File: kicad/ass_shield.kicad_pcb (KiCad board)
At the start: 2 copper layers, 80 x 80 mm, 151 parts, among them J1 6-40V, J2 DEBUG, J3 5V, J4 UART2, J5 U.FL, J6 i2s, J7 SP, J8 U.FL, M1 CR1220SMD, Q1 BC817, U1 OPiZero, U2 DS3231M, U3 24LC256, U4 nRF24L01P, U5 PCF8574, U6 CC2530F, X1 USB_F1, X2 USB_F1, Y1 9,84375 MHz, Y2 13,5600 MHz, Y3 4,8970 MHz, Y4 6,7458 MHz, Y5 32 MHz, Y6 16 MHz, Y7 32 MHz

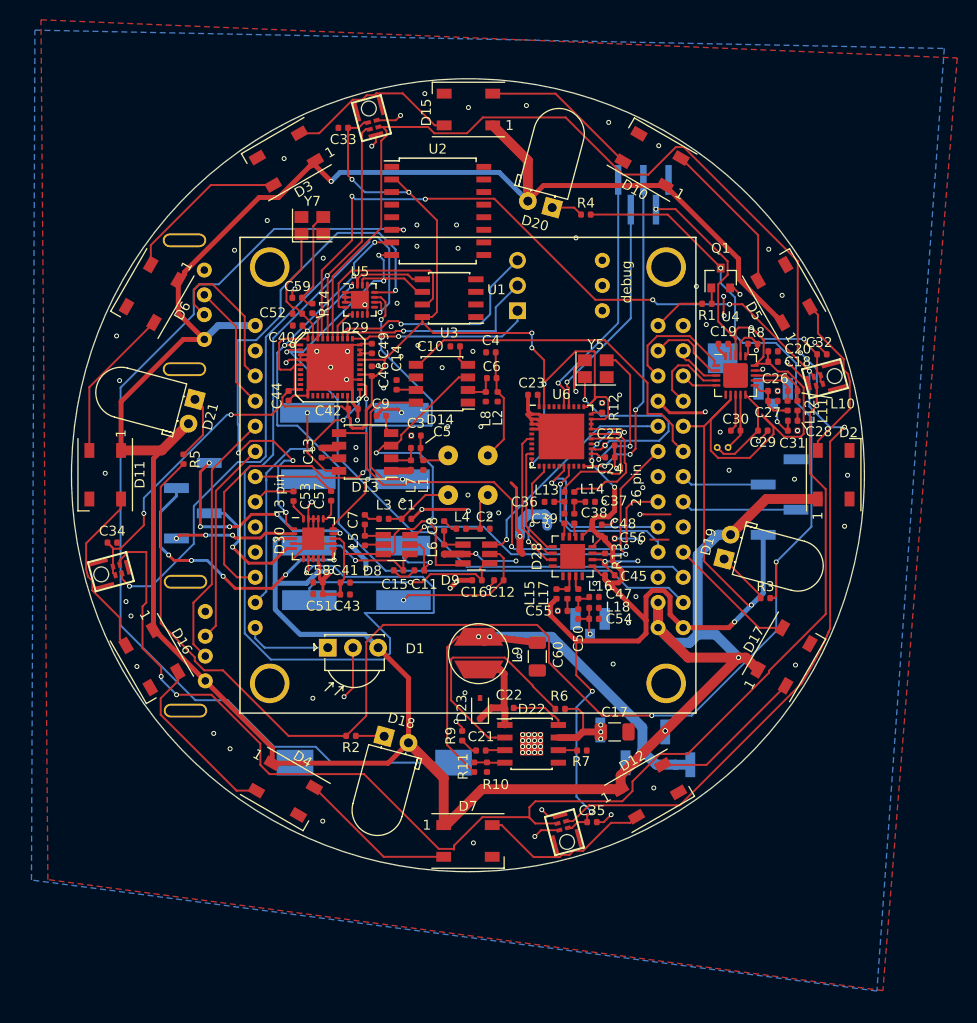
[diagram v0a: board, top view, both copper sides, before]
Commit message: a msg
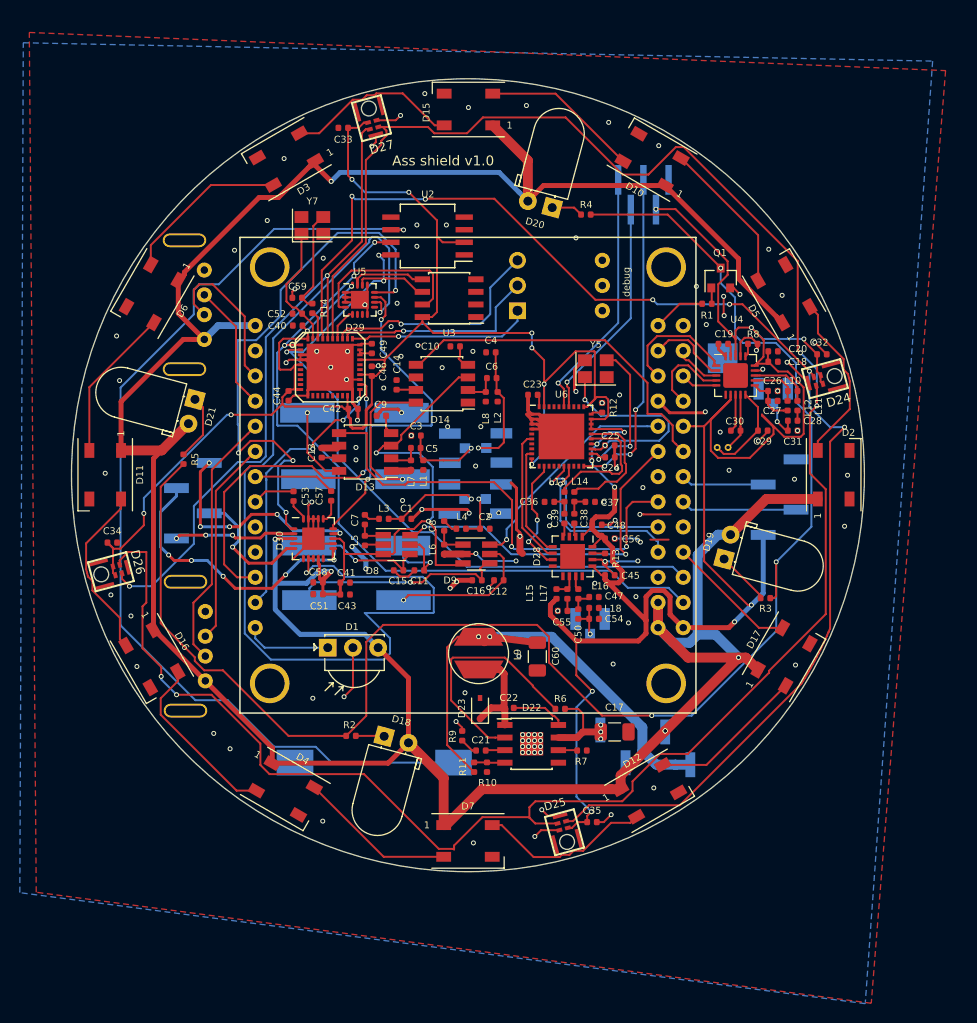
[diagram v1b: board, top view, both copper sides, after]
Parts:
- AE1, AE2, AE3, AE4: footprint imm:rf_antenna_0.8mm -> Connector_Coaxial:U.FL_Hirose_U.FL-R-SMT-1_Vertical; moved to B.Cu
- C10, C9: value 0,047 µF -> 47 nF
- C17: value 10µF 50V -> 10 µF 50V
- C22: value 100 nF -> 0,1 µF
- C60: value 22µF 6,3V -> 22 µF 6,3V
- D24, D25, D26, D27: value >VALUE -> ADMP421
- R1: value 200 -> 200 R
- R14: value 100 -> 100 R
- R2, R3, R4, R5: value 37 -> 37 R
- U2: footprint Package_SO:SOIC-16W_7.5x10.3mm_P1.27mm -> Package_SO:SO-8_5.3x6.2mm_P1.27mm
- moved U2 2.73 mm to (95.9, 75.9), turned to 180 degrees
- moved AE2 1.17 mm to (102.9, 97.2)
- moved AE1 0.97 mm to (98.7, 97.3), turned to 180 degrees
- moved AE4 0.94 mm to (102.8, 102.4)
- moved AE3 0.72 mm to (98.6, 102.4), turned to 180 degrees
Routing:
- net GND: track 183.3 -> 177.8 mm, vias 127 -> 126
- net Net-(AE1-Pad1): track 5.34 -> 8.59 mm, vias 0 -> 1
- net Net-(AE3-Pad1): track 6.99 -> 10.2 mm, vias 0 -> 1
- net Net-(AE2-Pad1): track 11.4 -> 13.0 mm, vias 0 -> 1
- net 3,3V: track 358.0 -> 358.8 mm
- net Net-(D28-Pad7): track 11.5 -> 12.0 mm
- net Net-(AE4-Pad1): track 5.15 -> 5.18 mm, vias 0 -> 1
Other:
- board text added: "Ass shield v1.0"
